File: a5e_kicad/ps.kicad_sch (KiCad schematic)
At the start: 52 parts, among them U15 SIC931BED-T1-GE3

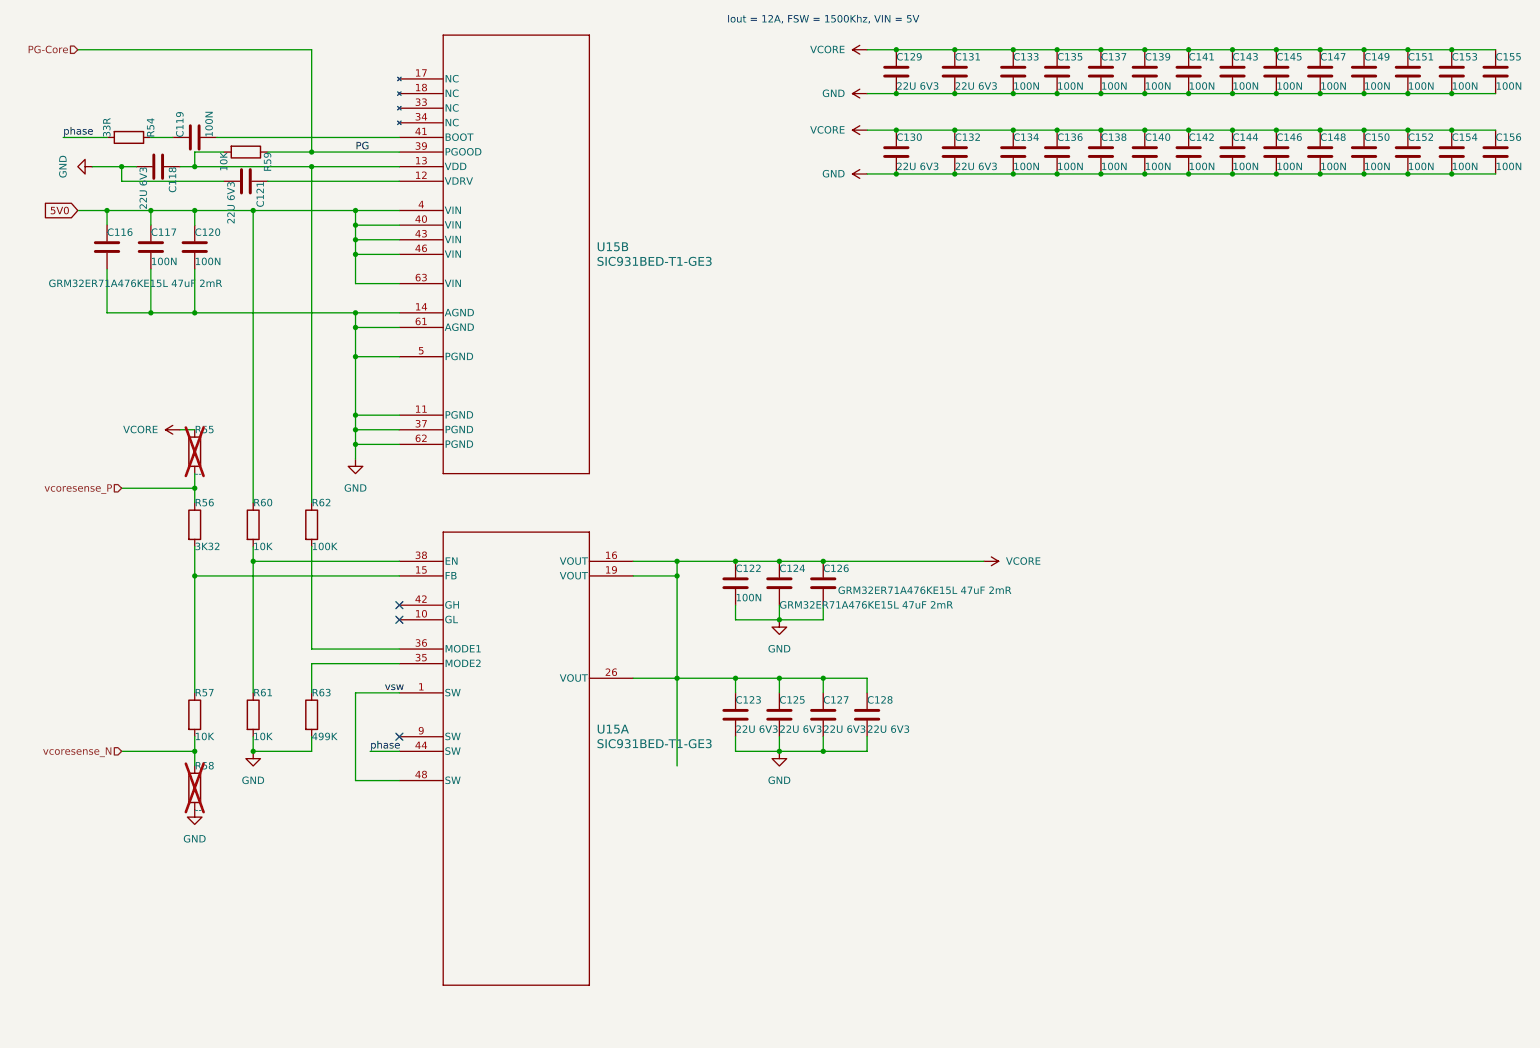
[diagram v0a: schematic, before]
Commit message: add comments
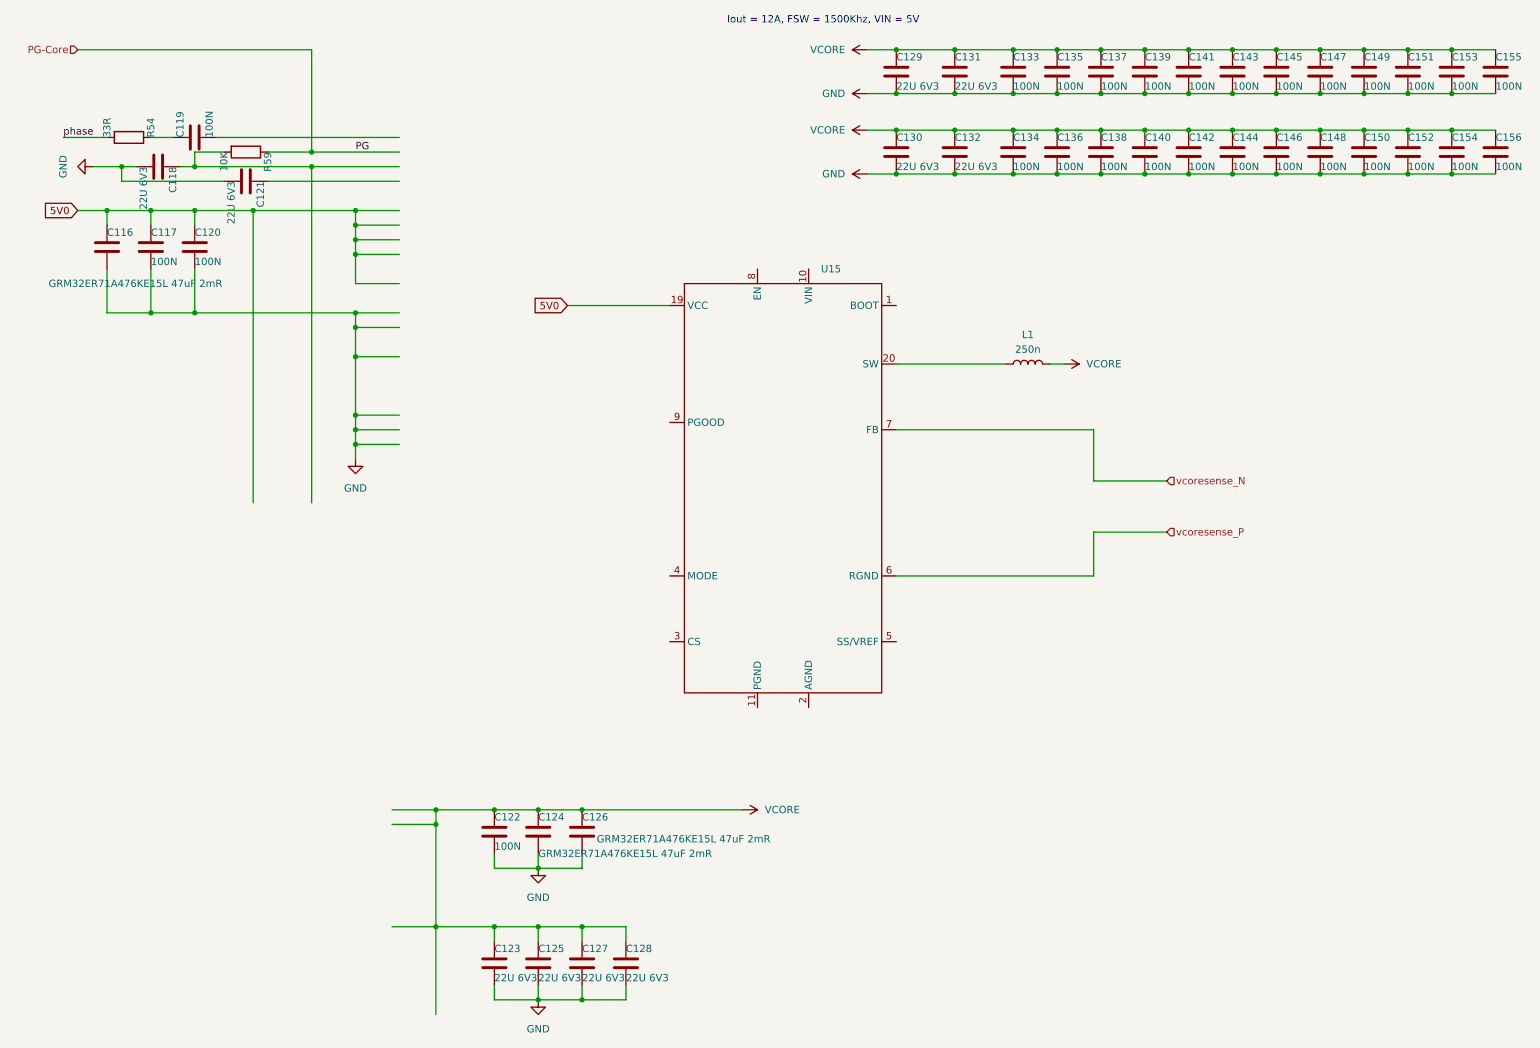
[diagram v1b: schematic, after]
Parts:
- removed R55, R58: --, Resistor_SMD:R_0402_1005Metric, symbol Device:R
- removed R56: 3K32, Resistor_SMD:R_0402_1005Metric, symbol Device:R
- removed R57, R60, R61: 10K, Resistor_SMD:R_0402_1005Metric, symbol Device:R
- removed R62: 100K, Resistor_SMD:R_0402_1005Metric, symbol Device:R
- removed R63: 499K, Resistor_SMD:R_0402_1005Metric, symbol Device:R
- removed U15: SIC931BED-T1-GE3, symbol SiC931bed:SIC931BED-T1-GE3
- added L1: 250n, agilex_lib:CMLE051H, symbol Device:L
- added U15: (no value), agilex_lib:TDA38812, symbol agilex_5_lib:TDA38812
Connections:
- net 5V0: now also U15.19 (VCC)
- net VCORE: now also L1.2
- net vcoresense_N: now also U15.7 (FB)
- net vcoresense_P: now also U15.6 (RGND)
- new net: L1.1, U15.20 (SW)
- no-connect marks 3 -> 0
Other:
- moved on the sheet: C122, C123, C124, C125, C126, C127, C128
